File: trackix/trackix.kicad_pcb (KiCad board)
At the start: 2 copper layers, 85.1 x 43.2 mm, 47 parts, among them IC1 SIM808, J1 GSM, J2 GPS, J3 SIM SLOT, J4 AVR-ISP-6, Q1 2N3904, Q2 2N3904, U1 ATmega328P-AU, U2 SIM-ST-MFF2

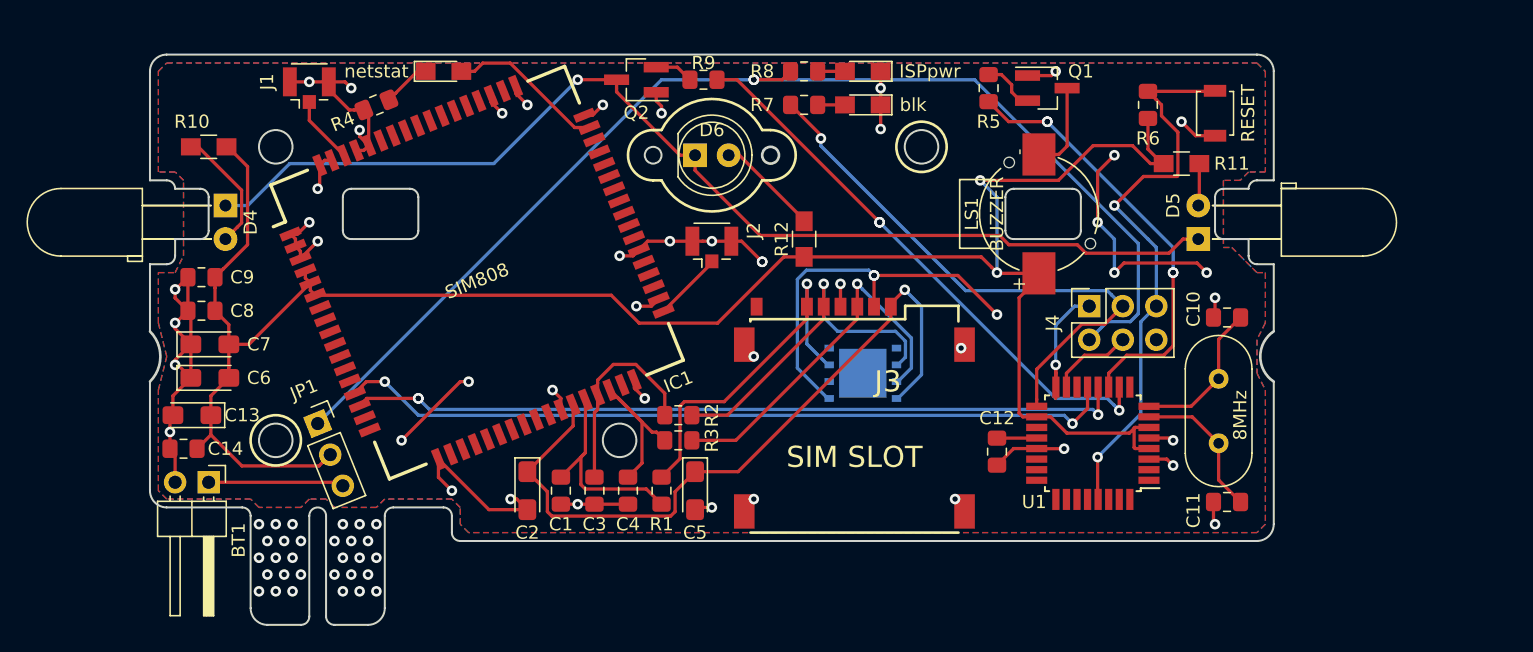
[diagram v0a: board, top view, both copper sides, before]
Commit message: all things so far
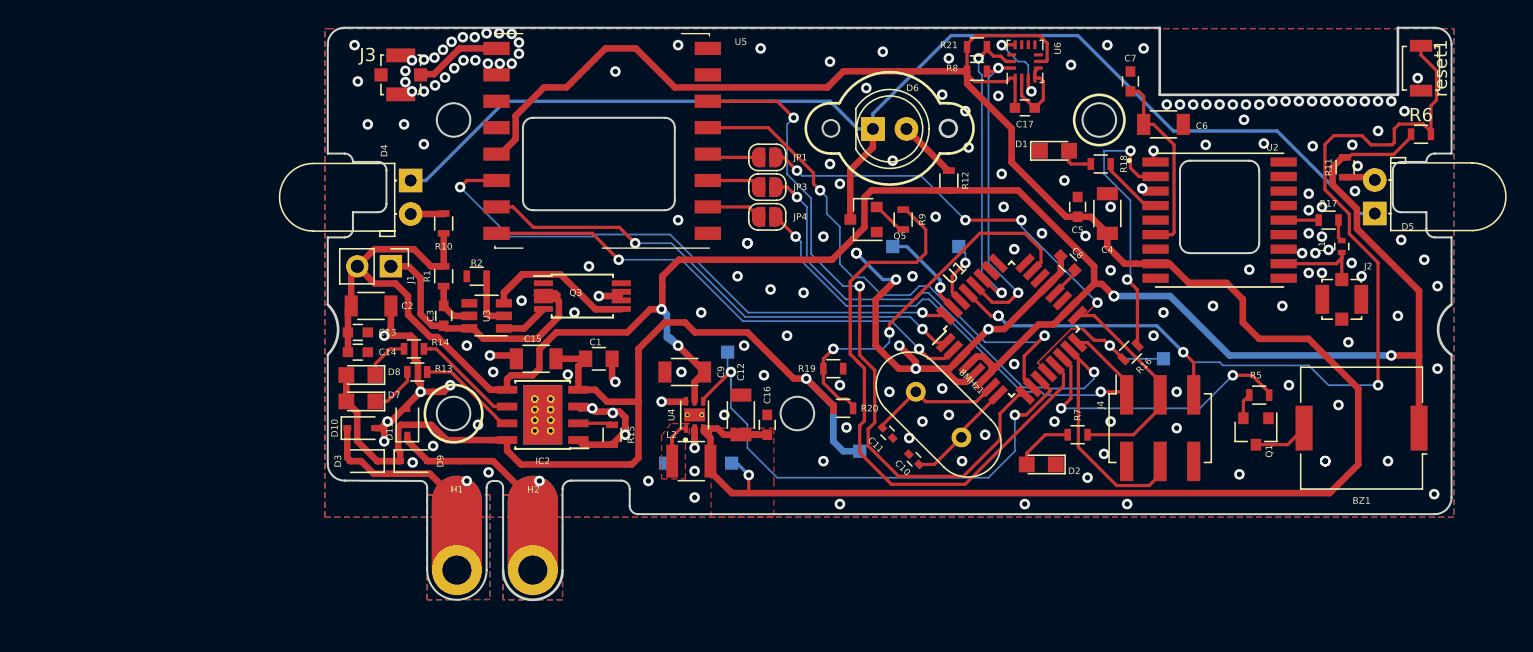
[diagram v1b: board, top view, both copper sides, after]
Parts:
- removed 8MHz: Crystal, Crystals:Crystal_HC49-4H_Vertical
- removed BT1: Li-Ion 3,7v, Connector_PinHeader_2.54mm:PinHeader_1x02_P2.54mm_Horizontal
- removed IC1: SIM808, QFN100P2400X2400X260-68N
- removed ISPpwr: ISP led, LEDs:LED_0805_HandSoldering
- removed LS1: BUZZER, CUI_CBT-09427-SMT
- removed Q2: 2N3904, Package_TO_SOT_SMD:SOT-23_Handsoldering
- removed R3: 22, Resistor_SMD:R_0805_2012Metric_Pad1.15x1.40mm_HandSolder
- removed R4: 470, Resistor_SMD:R_0805_2012Metric_Pad1.15x1.40mm_HandSolder
- removed RESET: reset, Buttons_Switches_SMD:SW_SPST_B3U-1000P
- removed blk: led 13, LEDs:LED_0805_HandSoldering
- removed netstat: netstat LED, LEDs:LED_0805_HandSoldering
- added 8MHz1: Crystal, Crystals:Crystal_HC49-U_Vertical, F.Cu at (106.2, 63.0)
- added BZ1: Buzzer, Buzzers_Beepers:Buzzer_Murata_PKMCS0909E4000-R1, F.Cu at (140.0, 65.8)
- added C15: 10uF, Capacitors_SMD:C_1206, F.Cu at (77.5, 60.5)
- added C16: 100nF, Capacitors_SMD:C_0603, F.Cu at (95.0, 65.5)
- added C17: C_100nF, Capacitors_SMD:C_0603, F.Cu at (114.5, 41.5)
- added D1: GPS_LED, LEDs:LED_0805, F.Cu at (116.8, 44.8)
- added D10: D_B5818WS SK, Diodes_SMD:D_SOD-323, F.Cu at (64.2, 65.8)
- added D11: D_B5818WS SK, Diodes_SMD:D_SOD-323, F.Cu at (67.8, 65.3)
- added D2: led 13, LEDs:LED_0805, F.Cu at (115.8, 68.5)
- added D3: D_B5818WS SK, Diodes_SMD:D_SOD-323, F.Cu at (64.5, 68.2)
- added D7: LED_chrg, LEDs:LED_0805, F.Cu at (64.2, 63.7)
- added D8: LED_stdby, LEDs:LED_0805, F.Cu at (64.2, 61.7)
- added D9: D_B5818WS SK, Diodes_SMD:D_SOD-323, F.Cu at (68.2, 68.2)
- added H1: DYNAMO_A, Mounting_Holes:MountingHole_2.2mm_M2_ISO14580_Pad, F.Cu at (71.5, 76.5)
- added H2: DYNAMO_B, Mounting_Holes:MountingHole_2.2mm_M2_ISO14580_Pad, F.Cu at (77.2, 76.5)
- added IC2: TP4056, Housings_SOIC:HTSOP-8-1EP_3.9x4.9mm_Pitch1.27mm_ThermalVias_LargeCopper, F.Cu at (78.0, 64.8)
- added JP3: MOSI, Jumper:SolderJumper-2_P1.3mm_Open_RoundedPad1.0x1.5mm, F.Cu at (95.0, 47.5)
- added JP4: MISO, Jumper:SolderJumper-2_P1.3mm_Open_RoundedPad1.0x1.5mm, F.Cu at (95.0, 49.8)
- added L1: L27nH, Inductors_SMD:L_0402, F.Cu at (138.5, 52.0)
- added L2: L2.2uH, Inductors_SMD:L_1210, F.Cu at (89.2, 68.2)
- added Q3: FS8205A, Housings_SSOP:TSSOP-8_4.4x3mm_Pitch0.65mm, F.Cu at (81.0, 55.8)
- added Q5: 2N3904, TO_SOT_Packages_SMD:SOT-23, F.Cu at (102.3, 50.0)
- added R13: 470, Resistors_SMD:R_0603, F.Cu at (68.5, 61.5)
- added R14: 470, Resistors_SMD:R_0603, F.Cu at (68.2, 59.8)
- added R15: 4k for Ibat 300mA, Resistors_SMD:R_0603, F.Cu at (83.2, 66.2)
- added R16: R100, Resistors_SMD:R_0603, F.Cu at (122.5, 60.0)
- added R17: R22, Resistors_SMD:R_0603, F.Cu at (137.5, 50.0)
- added R18: R100, Resistors_SMD:R_0603, F.Cu at (120.2, 45.8)
- added R19: R5k, Resistors_SMD:R_0603, F.Cu at (100.0, 61.2)
- added R20: R10k, Resistors_SMD:R_0603, F.Cu at (100.8, 64.2)
- added R21: 4.7k, Resistors_SMD:R_0603, F.Cu at (110.9, 36.9)
- added TP1: DYNAMO_A, Connectors_TestPoints:Test_Point_Pad_1.0x1.0mm, B.Cu at (71.5, 72.2)
- added TP2: DYNAMO_B, Connectors_TestPoints:Test_Point_Pad_1.0x1.0mm, B.Cu at (77.2, 72.2)
- added TP3: GND, Connectors_TestPoints:Test_Point_Pad_1.0x1.0mm, B.Cu at (87.3, 68.4)
- added TP4: VCC_IN_DC, Connectors_TestPoints:Test_Point_Pad_1.0x1.0mm, B.Cu at (102.0, 67.5)
- added TP5: AUX_ON, Connectors_TestPoints:Test_Point_Pad_1.0x1.0mm, B.Cu at (92.0, 60.0)
- added TP6: GPS_TX, Connectors_TestPoints:Test_Point_Pad_1.0x1.0mm, B.Cu at (125.0, 60.5)
- added TP7: TX, Connectors_TestPoints:Test_Point_Pad_1.0x1.0mm, B.Cu at (109.5, 52.0)
- added TP8: RX, Connectors_TestPoints:Test_Point_Pad_1.0x1.0mm, B.Cu at (104.5, 52.0)
- added TP9: TestPoint3.3V, Connectors_TestPoints:Test_Point_Pad_1.0x1.0mm, B.Cu at (92.3, 68.4)
- added U3: DW-01, TO_SOT_Packages_SMD:TSOT-23-6, F.Cu at (73.8, 57.2)
- added U4: TPS62291DRVR, user_added_kicad_libs:SON65P200X200X80-7N, F.Cu at (89.5, 64.8)
- added U5: RFM95W-868S2, RF_Modules:Hopref_RFM9XW_SMD, F.Cu at (82.5, 44.0)
- added U6: ADXL345BCCZ, Housings_LGA:Bosch_LGA-14_3x2.5mm_Pitch0.5mm, F.Cu at (114.5, 38.0)
- added reset1: reset, Buttons_Switches_SMD:SW_SPST_B3U-1000P, F.Cu at (144.5, 38.5)
- C1: value 22pF -> 100nF; footprint Capacitor_SMD:C_0805_2012Metric_Pad1.15x1.40mm_HandSolder -> Capacitors_SMD:C_0805
- C10, C11: footprint Capacitor_SMD:C_0805_2012Metric_Pad1.15x1.40mm_HandSolder -> Capacitors_SMD:C_0402
- C12: value 0,1uF -> 10uF; footprint Capacitor_SMD:C_0805_2012Metric_Pad1.15x1.40mm_HandSolder -> Capacitors_SMD:C_1206
- C13: footprint Capacitor_Tantalum_SMD:CP_EIA-3216-10_Kemet-I_Pad1.58x1.35mm_HandSolder -> Capacitors_SMD:C_0603
- C14: value 0,1uF -> 0.1uF; footprint Capacitor_SMD:C_0805_2012Metric_Pad1.15x1.40mm_HandSolder -> Capacitors_SMD:C_0603
- C2: value 1uF -> 10uF; footprint Capacitor_Tantalum_SMD:CP_EIA-3216-10_Kemet-I_Pad1.58x1.35mm_HandSolder -> Capacitors_SMD:C_1206
- C3: value 22pF -> C_100nF; footprint Capacitor_SMD:C_0805_2012Metric_Pad1.15x1.40mm_HandSolder -> Capacitors_SMD:C_0603
- C4: value 22pF -> C_4.7uF; footprint Capacitor_SMD:C_0805_2012Metric_Pad1.15x1.40mm_HandSolder -> Capacitors_SMD:C_1206
- C5: value 1uF -> C_100nF; footprint Capacitor_Tantalum_SMD:CP_EIA-3216-10_Kemet-I_Pad1.58x1.35mm_HandSolder -> Capacitors_SMD:C_0603
- C6: value 100uF -> C_4.7uF; footprint Capacitor_Tantalum_SMD:CP_EIA-3216-10_Kemet-I_Pad1.58x1.35mm_HandSolder -> Capacitors_SMD:C_1206
- C7: value 10uF -> C_100nF; footprint Capacitor_Tantalum_SMD:CP_EIA-3216-10_Kemet-I_Pad1.58x1.35mm_HandSolder -> Capacitors_SMD:C_0603
- C8: value 33pF -> 100nF; footprint Capacitor_SMD:C_0805_2012Metric_Pad1.15x1.40mm_HandSolder -> Capacitors_SMD:C_0603
- C9: value 10pF -> 10uF; footprint Capacitor_SMD:C_0805_2012Metric_Pad1.15x1.40mm_HandSolder -> Capacitors_SMD:C_1206
- D4, D5: footprint LED_THT:LED_D5.0mm_Horizontal_O6.35mm_Z15.0mm -> LEDs:LED_D5.0mm_Horizontal_O1.27mm_Z3.0mm
- D6: footprint LED_THT:LED_D5.0mm_FlatTop -> LEDs:LED_D5.0mm
- J1: value GSM -> BATTERY; footprint Connector_Coaxial:U.FL_Hirose_U.FL-R-SMT-1_Vertical -> Pin_Headers:Pin_Header_Straight_1x02_Pitch2.54mm
- J2: footprint Connector_Coaxial:U.FL_Hirose_U.FL-R-SMT-1_Vertical -> Connectors_Molex:Molex_Microcoaxial_RF
- J3: value SIM SLOT -> LORA_868; footprint SIM7100-6-1-15-00-X_REVA:GCT_SIM7100-6-1-15-00-X_REVA -> Connectors_Molex:Molex_Microcoaxial_RF
- J4: footprint Connector_PinSocket_2.54mm:PinSocket_2x03_P2.54mm_Vertical -> Socket_Strips:Socket_Strip_Straight_2x03_Pitch2.54mm_SMD
- JP1: value Power Selector -> SCK; footprint Connector_PinSocket_2.54mm:PinSocket_1x03_P2.54mm_Vertical -> Jumper:SolderJumper-2_P1.3mm_Open_RoundedPad1.0x1.5mm
- Q1: footprint Package_TO_SOT_SMD:SOT-23_Handsoldering -> TO_SOT_Packages_SMD:SOT-23
- R1: value 22 -> 100; footprint Resistor_SMD:R_0805_2012Metric_Pad1.15x1.40mm_HandSolder -> Resistors_SMD:R_0603
- R10, R11, R12: value 470 -> 330; footprint Resistors_SMD:R_0805_HandSoldering -> Resistors_SMD:R_0603
- R2: value 22 -> 1k; footprint Resistor_SMD:R_0805_2012Metric_Pad1.15x1.40mm_HandSolder -> Resistors_SMD:R_0603
- R5, R6, R9: footprint Resistor_SMD:R_0805_2012Metric_Pad1.15x1.40mm_HandSolder -> Resistors_SMD:R_0603
- R7: value 470 -> 330; footprint Resistor_SMD:R_0805_2012Metric_Pad1.15x1.40mm_HandSolder -> Resistors_SMD:R_0603
- R8: value 470 -> 4.7k; footprint Resistor_SMD:R_0805_2012Metric_Pad1.15x1.40mm_HandSolder -> Resistors_SMD:R_0603
- U1: footprint Package_QFP:TQFP-32_7x7mm_P0.8mm -> Housings_QFP:TQFP-32_7x7mm_Pitch0.8mm
- U2: value SIM-ST-MFF2 -> SIM28ML; footprint SIM-ST-MFF2:PSON127P500X600X82-9N -> SIM28ML:XCVR_SIM28ML; moved to F.Cu
- moved C6 74.7 mm to (125.0, 42.8)
- moved C7 72.5 mm to (122.5, 39.5), turned to 90 degrees
- moved C8 65.7 mm to (117.8, 53.2), turned to 315 degrees
- moved J2 47.9 mm to (138.5, 56.0), turned to 180 degrees
- moved J3 42.9 mm to (67.2, 39.0), turned to 90 degrees
- moved C4 41.9 mm to (120.8, 49.5), turned to 90 degrees
- moved JP1 39.6 mm to (95.0, 45.2), turned to 0 degrees
- moved C9 37.3 mm to (88.8, 61.5), turned to 180 degrees
- moved C5 36.1 mm to (118.5, 49.0), turned to 90 degrees
- moved R7 32.4 mm to (118.5, 66.2), turned to 0 degrees
- moved R5 31.0 mm to (132.2, 63.2), turned to 180 degrees
- moved Q1 30.4 mm to (132.0, 66.0), turned to 270 degrees
- moved U2 29.4 mm to (129.2, 50.0)
- moved C11 26.2 mm to (104.1, 66.1), turned to 135 degrees
- moved C10 26.0 mm to (106.1, 68.1), turned to 315 degrees
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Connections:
- net Net-(J4-Pad5) renamed RESET
- C1 pad 1: Net-(C1-Pad1) -> CHARGE_DETECT
- C12 pad 1: Net-(C12-Pad1) -> +3V3
- C2 pad 1: Net-(C2-Pad1) -> +BATT
- C3 pad 2: GND -> -BATT
- C4 pad 1: Net-(C4-Pad1) -> +3V3
- C5 pad 1: Net-(C2-Pad1) -> +3V3
- C6 pad 1: GND -> Net-(C6-Pad1)
- C6 pad 2: +BATT -> GND
- C7 pad 1: GND -> Net-(C6-Pad1)
- C7 pad 2: +BATT -> GND
- C8 pad 2: +BATT -> Net-(C8-Pad2)
- C9 pad 1: GND -> +BATT
- C9 pad 2: +BATT -> GND
- J1 pad 1: Net-(IC1-Pad66) -> -BATT
- J1 pad 2: GND -> +BATT
- J2 pad 1: Net-(IC1-Pad35) -> Net-(J2-Pad1)
- J3 pad 1: (no net) -> Net-(J3-Pad1)
- J3 pad 2: (no net) -> GND
- JP1 pad 1: Net-(J4-Pad2) -> SCK
- JP1 pad 2: +BATT -> Net-(J4-Pad3)
- R1 pad 1: Net-(J3-PadC7) -> Net-(C3-Pad1)
- R1 pad 2: Net-(C1-Pad1) -> +BATT
- R2 pad 1: Net-(J3-PadC3) -> Net-(R2-Pad1)
- R2 pad 2: Net-(C3-Pad1) -> GND
- R5 pad 1: Net-(R5-Pad1) -> DRIVE_BUZZER
- R8 pad 1: Net-(J4-Pad2) -> +3V3
- R8 pad 2: Net-(D3-Pad2) -> SCL
- R9 pad 1: Net-(R9-Pad1) -> DRIVE_LED
- U1 pad 1: Net-(U1-Pad1) -> DIO_1
- U1 pad 10: Net-(R9-Pad1) -> NSS
- U1 pad 11: Net-(R5-Pad1) -> AUX_ON
- U1 pad 12: simRX -> GPS_TX
- U1 pad 13: simTX -> DRIVE_LED
- U1 pad 14: Net-(U1-Pad14) -> DRIVE_BUZZER
- U1 pad 2: Net-(U1-Pad2) -> DIO_2
- U1 pad 20: Net-(C12-Pad1) -> Net-(C8-Pad2)
- U1 pad 27: Net-(U1-Pad27) -> SDA
- U1 pad 28: Net-(U1-Pad28) -> SCL
- U1 pad 32: Net-(U1-Pad32) -> DIO_0
- U1 pad 9: Net-(U1-Pad9) -> RFM_RESET
- U2 pad 2: (no net) -> Net-(R16-Pad1)
- U2 pad 3: Net-(J3-PadC7) -> GND
- U2 pad 4: (no net) -> Net-(R18-Pad2)
- U2 pad 5: (no net) -> Net-(U2-Pad5)
- U2 pad 6: Net-(J3-PadC3) -> Net-(C6-Pad1)
- U2 pad 7: Net-(J3-PadC2) -> Net-(U2-Pad7)
- U2 pad 8: Net-(C2-Pad1) -> +3V3
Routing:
- net +3V3: track 0.00 -> 176.5 mm, vias 0 -> 1
- net Net-(J4-Pad2): track 90.9 -> 0.00 mm, vias 2 -> 0
- net GND: track 169.2 -> 82.2 mm, vias 44 -> 174
- net CHARGE_DETECT: track 0.00 -> 84.1 mm, vias 0 -> 1
- net simTX: track 59.2 -> 0.00 mm, vias 2 -> 0
- net simRX: track 58.7 -> 0.00 mm, vias 3 -> 0
- net DRIVE_LED: track 0.00 -> 58.5 mm
- net Net-(C2-Pad1): track 55.6 -> 0.00 mm, vias 1 -> 0
- net RFM_RESET: track 0.00 -> 52.3 mm, vias 0 -> 2
- net Net-(J4-Pad4): track 6.37 -> 52.9 mm, vias 0 -> 2
- net DIO_0: track 0.00 -> 44.2 mm, vias 0 -> 2
- net Net-(R9-Pad1): track 42.6 -> 0.00 mm, vias 3 -> 0
- net AUX_ON: track 0.00 -> 41.7 mm, vias 0 -> 2
- net NSS: track 0.00 -> 40.7 mm, vias 0 -> 2
- net DIO_1: track 0.00 -> 38.8 mm, vias 0 -> 2
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- added copper zone on F.Cu, net +3V3
- added copper zone on B.Cu, net DYNAMO_A
- added copper zone on F.Cu, net DYNAMO_A
- added copper zone on B.Cu, net DYNAMO_B
- added copper zone on F.Cu, net DYNAMO_B
- added copper zone on F.Cu, net GND
- added copper zone on F.Cu, net Net-(L2-Pad1)
- removed copper zone on F.Cu, net +BATT
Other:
- board size 85.1 x 43.2 mm -> 85.1 x 43.3 mm
- rule trace_min: 0.2 -> 0.1
- board text added: "3.3V"
- board text added: "AUX EN"
- board text added: "GND"
- board text added: "GPS ANTENNA LOCATION"
- board text added: "GPS TX"
- board text added: "RX"
- board text added: "TX"
- board text added: "VCC DC"
- board text added: "trackix V_0.2 2020-05-04"
- board text removed: "trackix v.0.1 2019-02-18"
